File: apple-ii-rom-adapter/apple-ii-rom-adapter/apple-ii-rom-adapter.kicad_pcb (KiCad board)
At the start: 2 copper layers, 51.6 x 43.9 mm, 12 parts, among them J1 ROMSEL, J2 9316 insert, J3 74LS138 insert, U1 28C256, U2 74LS20, U3 74LS138, U4 74LS02

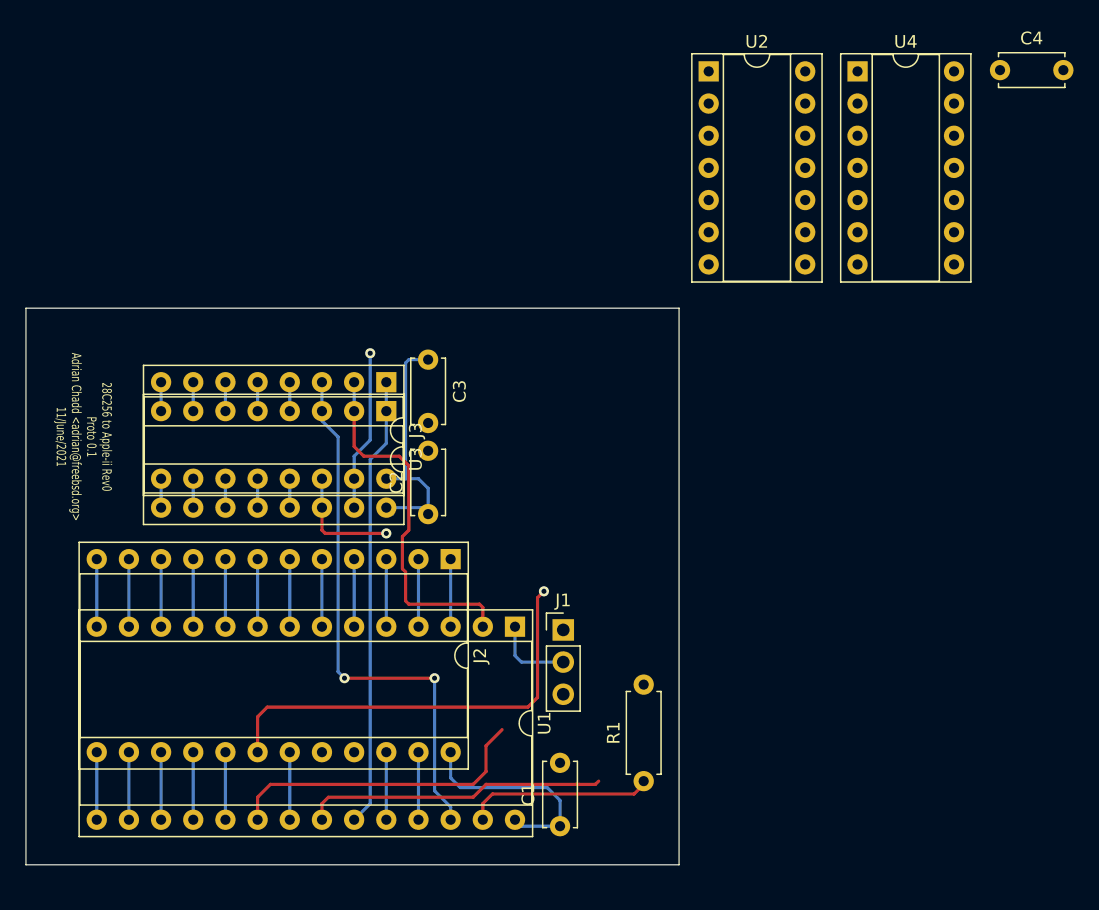
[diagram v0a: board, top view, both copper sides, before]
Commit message: Rom adapter update
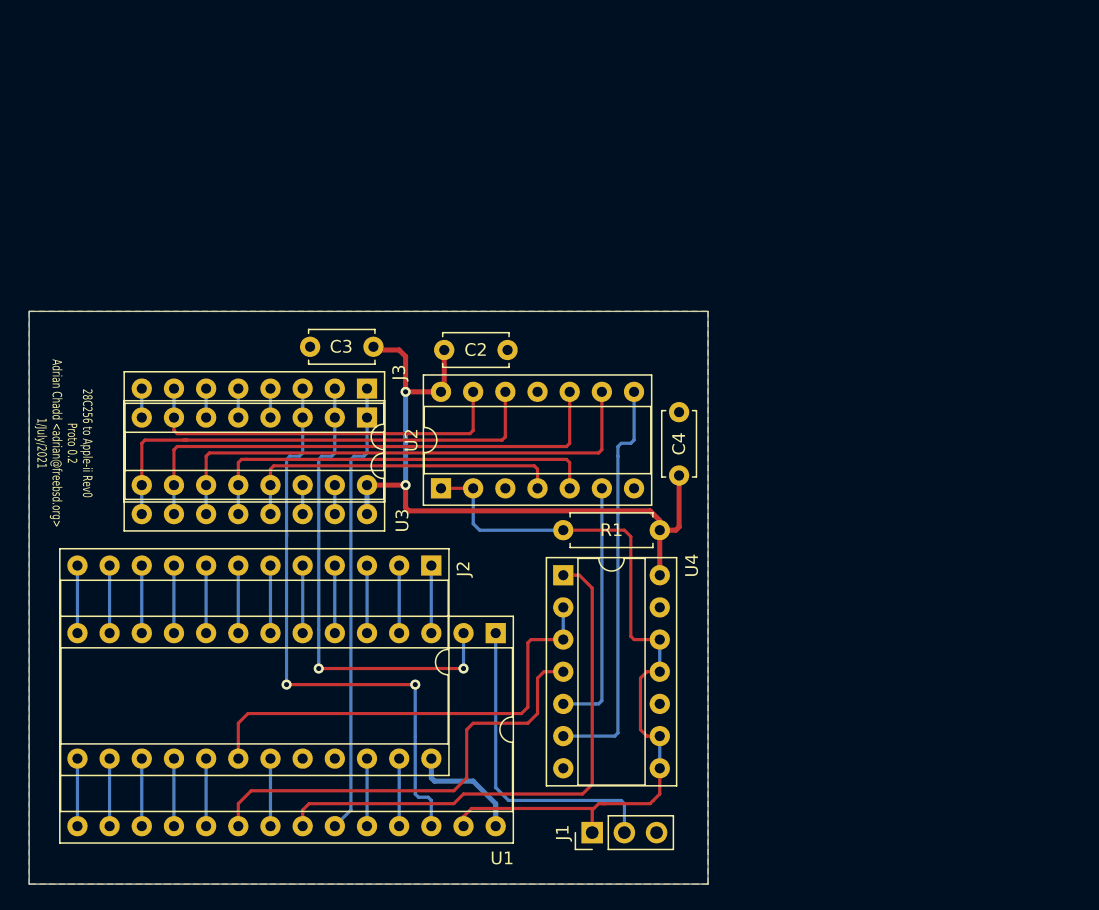
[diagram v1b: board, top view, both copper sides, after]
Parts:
- removed C1: 0.1uF, Capacitor_THT:C_Disc_D5.0mm_W2.5mm_P5.00mm
- moved U4 46.1 mm to (54.4, 33.0)
- moved C4 40.8 mm to (63.5, 25.1), turned to 90 degrees
- moved U2 39.1 mm to (44.7, 26.2), turned to 90 degrees
- moved R1 20.8 mm to (54.4, 29.5), turned to 0 degrees
- moved J1 16.2 mm to (56.6, 53.3), turned to 90 degrees
- moved C2 13.0 mm to (45.0, 15.2), turned to 0 degrees
- moved C3 4.44 mm to (39.4, 15.0), turned to 180 degrees
- moved J2 1.61 mm to (43.9, 32.3)
- moved U3 1.61 mm to (38.9, 20.6)
- moved J3 1.61 mm to (38.9, 18.3)
- moved U1 1.61 mm to (49.0, 37.6)
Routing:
- net SOFT_5: track 14.6 -> 63.1 mm
- net A_SEL_5: track 2.29 -> 40.6 mm
- net A_SEL_4: track 2.29 -> 40.6 mm
- net A_SEL_6: track 2.29 -> 38.3 mm
- net Net-(U2-Pad8): track 0.00 -> 32.6 mm
- net A_SEL_3: track 2.29 -> 32.7 mm
- net A_SEL_7: track 2.29 -> 30.2 mm
- net VCC: track 38.5 -> 66.3 mm, vias 0 -> 2
- net A_SEL_2: track 2.29 -> 26.4 mm
- net Net-(U2-Pad6): track 0.00 -> 19.9 mm
- net N_OE: track 24.1 -> 43.2 mm
- net A14: track 6.31 -> 25.2 mm
- net N_CS: track 24.5 -> 35.6 mm
- net A_SEL_0: track 12.7 -> 2.29 mm, vias 1 -> 0
- net A12: track 28.8 -> 37.3 mm, vias 0 -> 2
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- added copper zone on B.Cu, net GND
- added copper zone on F.Cu, net GND
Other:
- board size 51.6 x 43.9 mm -> 53.6 x 45.2 mm
- board text added: "28C256 to Apple-ii Rev0 Proto 0.2 Adrian Chadd <adrian@freebsd.org> 1/July/2021"
- board text removed: "28C256 to Apple-ii Rev0 Proto 0.1 Adrian Chadd <adrian@freebsd.org> 11/June/2021"
